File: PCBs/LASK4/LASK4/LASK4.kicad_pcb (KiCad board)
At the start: 2 copper layers, 16 parts, among them J1 Conn_01x02, U1 A1101ELHL, U2 A1101ELHL, U3 Charge37lion, U4 A1101ELHL, U5 A1101ELHL, U6 EPS32-S2-Mini

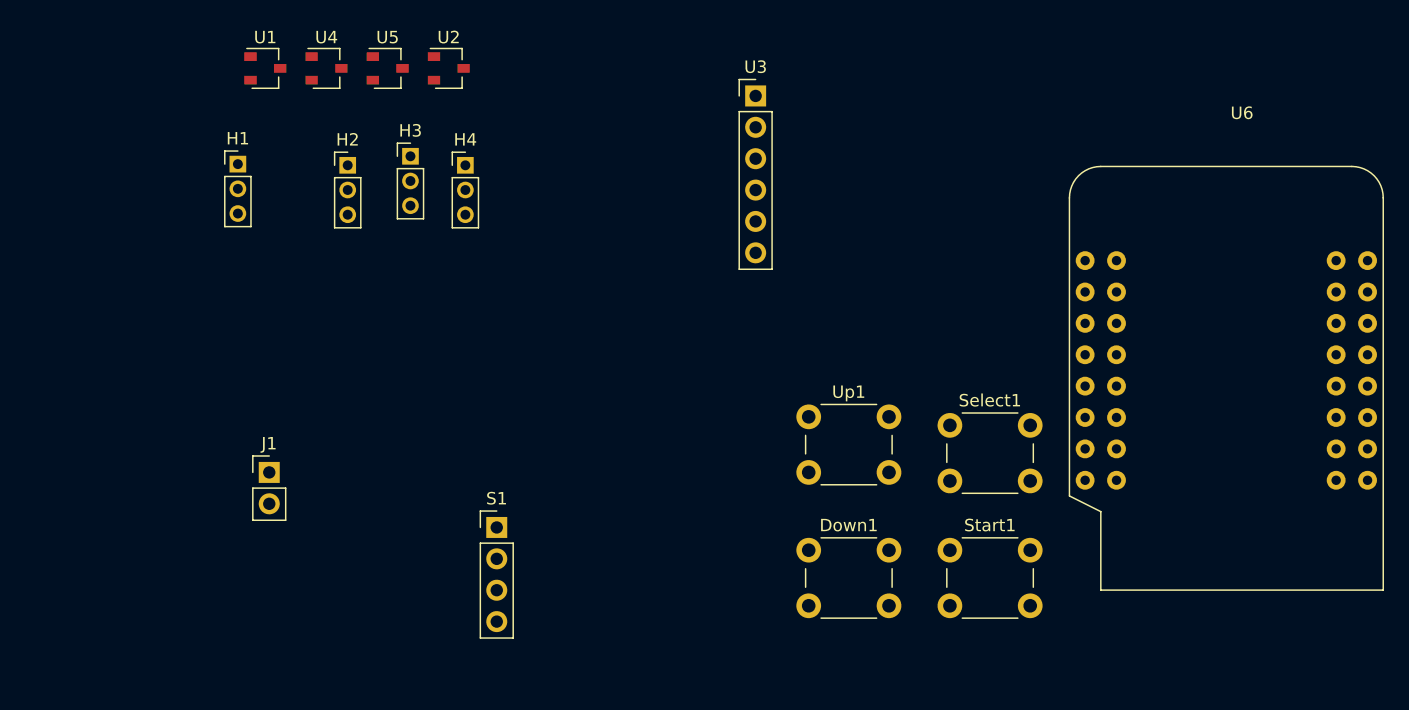
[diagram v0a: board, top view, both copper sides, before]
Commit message: LASK4 Update
Updated LASK4 PCB and pertaining documents.
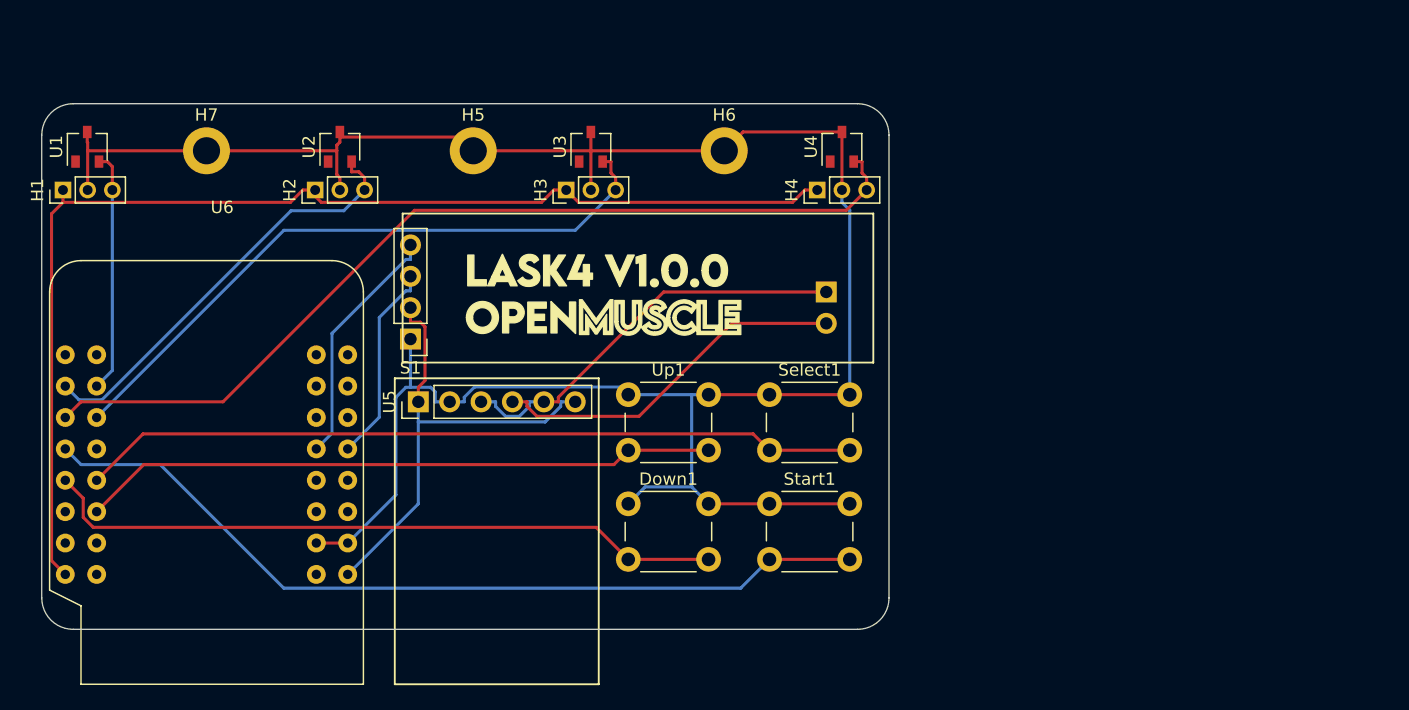
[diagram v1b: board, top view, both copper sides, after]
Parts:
- added H5: MountingHole_Pad, MountingHole:MountingHole_2.2mm_M2_DIN965_Pad, F.Cu at (168.9, 76.2)
- added H6: MountingHole_Pad, MountingHole:MountingHole_2.2mm_M2_DIN965_Pad, F.Cu at (189.2, 76.2)
- added H7: MountingHole_Pad, MountingHole:MountingHole_2.2mm_M2_DIN965_Pad, F.Cu at (147.3, 76.2)
- J1: moved to B.Cu
- U3: value Charge37lion -> A1101ELHL; footprint Connector_PinHeader_2.54mm:PinHeader_1x06_P2.54mm_Vertical -> Package_TO_SOT_SMD:SOT-23W
- U5: value A1101ELHL -> Charge37lion; footprint Package_TO_SOT_SMD:SOT-23W -> Connector_PinHeader_2.54mm:PinHeader_1x06_P2.54mm_Vertical
- moved U6 82.9 mm to (148.6, 81.3)
- moved J1 47.4 mm to (197.5, 87.6), turned to 180 degrees
- moved U4 42.2 mm to (198.8, 75.9), turned to 90 degrees
- moved H4 28.6 mm to (196.8, 79.4), turned to 90 degrees
- moved U5 27.1 mm to (164.5, 96.5), turned to 90 degrees
- moved S1 16.8 mm to (163.8, 91.4), turned to 180 degrees
- moved U1 15.8 mm to (137.7, 75.9), turned to 90 degrees
- moved Start1 15.1 mm to (192.9, 104.8)
- moved Down1 15.1 mm to (181.5, 104.8)
- moved Select1 14.8 mm to (192.9, 95.9)
- moved Up1 14.7 mm to (181.5, 95.9)
- moved H1 14.3 mm to (135.7, 79.4), turned to 90 degrees
- moved U3 14.0 mm to (178.4, 75.9), turned to 90 degrees
- moved H3 12.9 mm to (176.4, 79.4), turned to 90 degrees
- moved U2 10.9 mm to (158.1, 75.9), turned to 90 degrees
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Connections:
- U3 pad 1: +5V -> unconnected-(U3-Pad1)
- U3 pad 2: GND -> /GPIO_4_ADC1_3
- U3 pad 3: /BatGND -> GND
- U4 pad 2: /GPIO_4_ADC1_3 -> /GPIO_5_ADC1_4
- U5 pad 1: unconnected-(U5-Pad1) -> +5V
- U5 pad 2: /GPIO_5_ADC1_4 -> GND
- U5 pad 3: GND -> /BatGND
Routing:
- net GND: track 0.00 -> 183.1 mm
- net +3.3V: track 0.00 -> 95.6 mm
- net /GPIO_5_ADC1_4: track 0.00 -> 75.6 mm
- net /Start: track 0.00 -> 69.1 mm
- net /Select: track 0.00 -> 63.1 mm
- net /Down: track 0.00 -> 55.6 mm
- net /GPIO_4_ADC1_3: track 0.00 -> 52.8 mm
- net /Up: track 0.00 -> 51.6 mm
- net +5V: track 0.00 -> 38.7 mm
- net /GPIO_3_ADC1_2: track 0.00 -> 34.8 mm
- net /BatGND: track 0.00 -> 33.2 mm
- net /BatV3-7: track 0.00 -> 29.2 mm
- net /SDA34: track 0.00 -> 19.9 mm
- net /GPIO_2_ADC1_1: track 0.00 -> 19.5 mm
- net /SCL33: track 0.00 -> 16.3 mm
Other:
- board outline added: 68.6 x 42.5 mm
